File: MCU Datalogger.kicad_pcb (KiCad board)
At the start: 2 copper layers, 50.9 x 30.2 mm, 29 parts, among them J1 Conn_01x04_Pin, J2 Conn_01x09_Pin, J3 Conn_01x04_Pin, J4 Conn_02x03_Odd_Even, U1 24LC1025, U2 24LC1025, U3 DS1337S_, U4 ATMEGA328P-AU, Y1 32.768 KHz, Y2 16 MHz

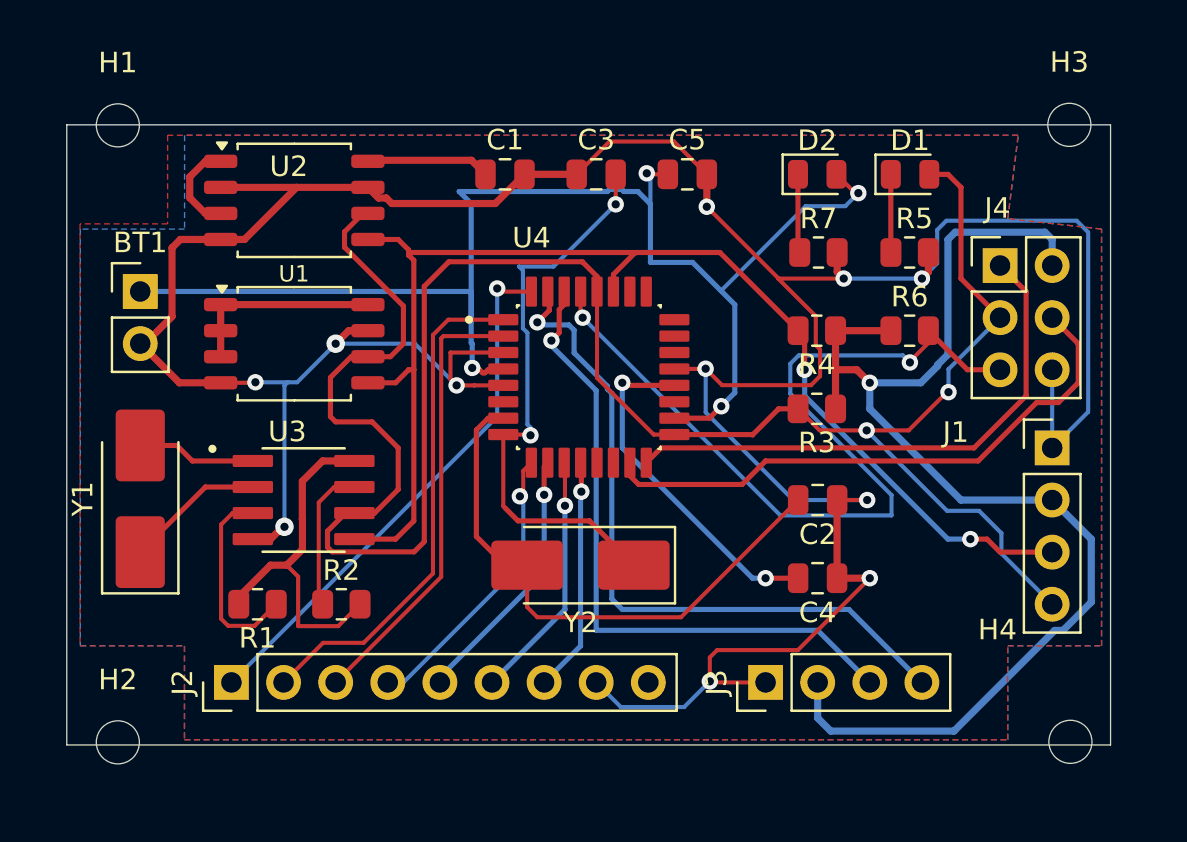
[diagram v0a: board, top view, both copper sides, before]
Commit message: Refined Routing Completed
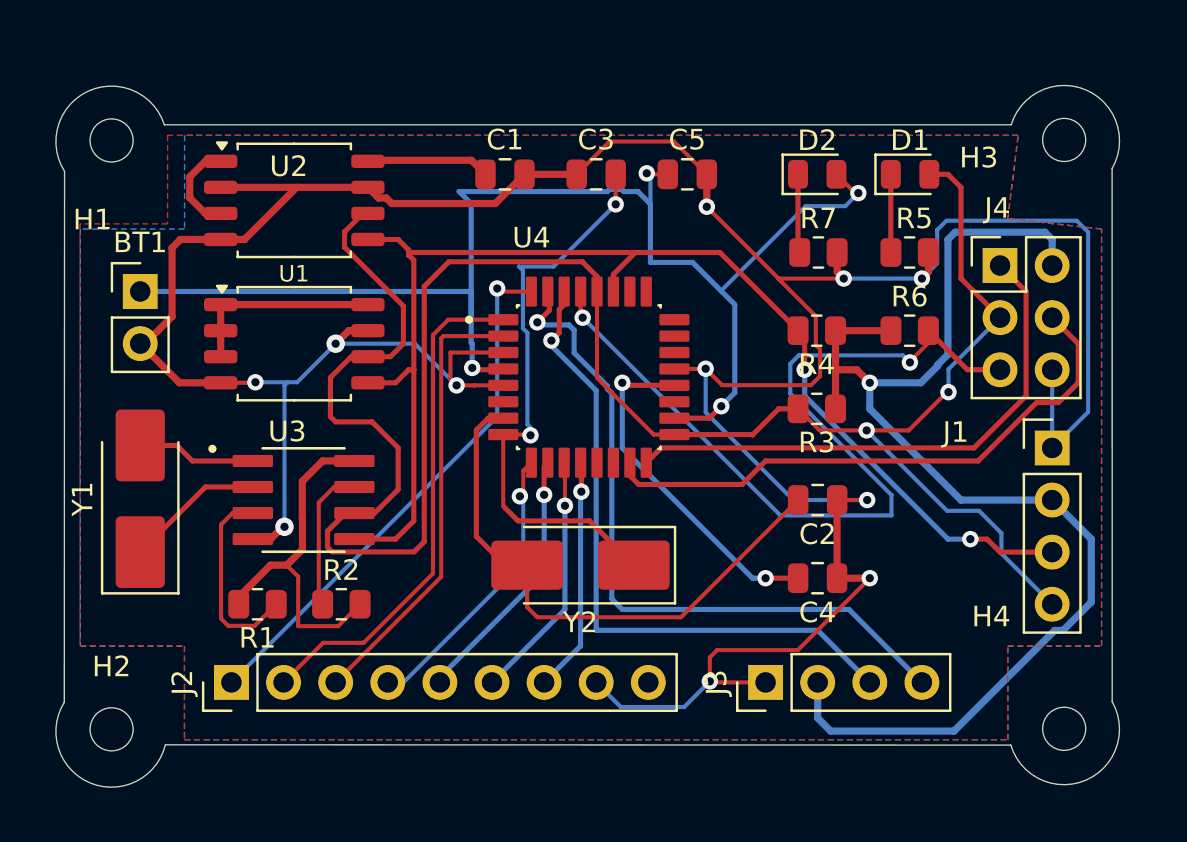
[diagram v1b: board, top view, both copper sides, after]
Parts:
- moved H1 0.80 mm to (66.5, 68.8)
- moved H3 0.78 mm to (113.0, 68.8)
- moved H2 0.70 mm to (66.5, 97.5)
- moved H4 0.70 mm to (113.0, 97.5)
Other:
- board size 50.9 x 30.2 mm -> 51.8 x 34.2 mm
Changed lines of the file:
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@@
 	(footprint "MountingHole:MountingHole_2.1mm"
 		(layer "F.Cu")
-		(at 66.8528 98.171)
+		(at 66.548 97.536)
 		(descr "Mounting Hole 2.1mm, no annular, generated by kicad-footprint-generator mountinghole.py")
 		(tags "mountinghole")
@@
 	(footprint "MountingHole:MountingHole_2.1mm"
 		(layer "F.Cu")
-		(at 113.284 98.1456)
+		(at 112.9792 97.5106)
 		(descr "Mounting Hole 2.1mm, no annular, generated by kicad-footprint-generator mountinghole.py")
 		(tags "mountinghole")
@@
 	(footprint "MountingHole:MountingHole_2.1mm"
 		(layer "F.Cu")
-		(at 66.8528 68.0974)
+		(at 66.548 68.834)
 		(descr "Mounting Hole 2.1mm, no annular, generated by kicad-footprint-generator mountinghole.py")
 		(tags "mountinghole")
 		(property "Reference" "H1"
-			(at 0 -3.05 0)
+			(at -0.928 3.866 0)
 			(layer "F.SilkS")
 			(effects
@@
 	(footprint "MountingHole:MountingHole_2.1mm"
 		(layer "F.Cu")
-		(at 113.2332 68.072)
+		(at 112.9792 68.8086)
 		(descr "Mounting Hole 2.1mm, no annular, generated by kicad-footprint-generator mountinghole.py")
 		(tags "mountinghole")
 		(property "Reference" "H3"
-			(at 0 -3.05 0)
+			(at -4.1592 0.8714 0)
 			(layer "F.SilkS")
 			(effects
@@
 		)
 	)
-	(gr_rect
-		(start 64.3636 68.072)
-		(end 115.240201 98.298)
+	(gr_line
+		(start 64.242154 96.219477)
+		(end 64.254954 70.341677)
+		(stroke
+			(width 0.05)
+			(type default)
+		)
+		(layer "Edge.Cuts")
+	)
+	(gr_arc
+		(start 64.254954 70.341677)
+		(mid 65.394627 66.437058)
+		(end 69.12 68.07)
+		(stroke
+			(width 0.05)
+			(type default)
+		)
+		(layer "Edge.Cuts")
+	)
+	(gr_arc
+		(start 69.17 98.29)
+		(mid 65.491502 100.145426)
+		(end 64.242152 96.219477)
+		(stroke
+			(width 0.05)
+			(type default)
+		)
+		(layer "Edge.Cuts")
+	)
+	(gr_line
+		(start 110.378307 98.305384)
+		(end 69.169999 98.29)
+		(stroke
+			(width 0.05)
+			(type default)
+		)
+		(layer "Edge.Cuts")
+	)
+	(gr_line
+		(start 115.316 70.2)
+		(end 115.32 96.190002)
+		(stroke
+			(width 0.05)
+			(type default)
+		)
+		(layer "Edge.Cuts")
+	)
+	(gr_line
+		(start 69.12 68.070003)
+		(end 110.396855 68.071052)
+		(stroke
+			(width 0.05)
+			(type default)
+		)
+		(layer "Edge.Cuts")
+	)
+	(gr_arc
+		(start 110.396855 68.071052)
+		(mid 114.051623 66.37391)
+		(end 115.316 70.2)
+		(stroke
+			(width 0.05)
+			(type default)
+		)
+		(layer "Edge.Cuts")
+	)
+	(gr_arc
+		(start 115.32 96.19)
+		(mid 114.034573 100.016923)
+		(end 110.378305 98.305384)
 		(stroke
 			(width 0.05)
 			(type default)
 		)
-		(fill no)
 		(layer "Edge.Cuts")
 	)
@@
 	)
 	(segment
-		(start 84.629801 80.159401)
-		(end 84.747221 80.159401)
+		(start 84.2148 80.01)
+		(end 85.6 80.01)
 		(width 0.25)
 		(layer "F.Cu")
@@
 	)
 	(segment
-		(start 84.4804 80.01)
-		(end 84.629801 80.159401)
-		(width 0.25)
-		(layer "F.Cu")
-		(net 1)
-	)
-	(segment
-		(start 84.2148 80.01)
-		(end 84.4804 80.01)
-		(width 0.25)
-		(layer "F.Cu")
-		(net 1)
-	)
-	(segment
-		(start 84.747221 80.159401)
-		(end 84.896622 80.01)
-		(width 0.25)
-		(layer "F.Cu")
-		(net 1)
-	)
-	(segment
 		(start 85.6 80.01)
 		(end 85.64 79.97)
@@
 	)
 	(segment
-		(start 84.896622 80.01)
-		(end 85.6 80.01)
-		(width 0.25)
-		(layer "F.Cu")
-		(net 1)
-	)
-	(segment
 		(start 92.6846 70.485)
 		(end 92.6338 70.4342)
@@
 	)
 	(segment
-		(start 90.932 91.186)
-		(end 91.44 91.694)
+		(start 87.4268 77.8256)
+		(end 88.83848 77.8256)
 		(width 0.25)
 		(layer "B.Cu")
@@
 	)
 	(segment
-		(start 87.2998 77.6986)
-		(end 87.4268 77.8256)
-		(width 0.25)
-		(layer "B.Cu")
-		(net 19)
-	)
-	(segment
-		(start 87.4268 77.8256)
-		(end 88.83848 77.8256)
+		(start 90.932 91.186)
+		(end 91.44 91.694)
 		(width 0.25)
 		(layer "B.Cu")
@@
 	)
 	(segment
-		(start 91.44 91.694)
-		(end 102.489 91.694)
+		(start 87.2998 77.6986)
+		(end 87.4268 77.8256)
 		(width 0.25)
 		(layer "B.Cu")
@@
 	)
 	(segment
-		(start 89.0926 79.18497)
-		(end 90.714 80.80637)
+		(start 102.489 91.694)
+		(end 106.045 95.25)
 		(width 0.25)
 		(layer "B.Cu")
@@
 	)
 	(segment
-		(start 102.489 91.694)
-		(end 106.045 95.25)
+		(start 90.932 81.16372)
+		(end 90.932 91.186)
 		(width 0.25)
 		(layer "B.Cu")
@@
 	)
 	(segment
-		(start 90.932 81.16372)
-		(end 90.932 91.186)
+		(start 91.44 91.694)
+		(end 102.489 91.694)
+		(width 0.25)
+		(layer "B.Cu")
+		(net 19)
+	)
+	(segment
+		(start 89.0926 79.18497)
+		(end 90.714 80.80637)
 		(width 0.25)
 		(layer "B.Cu")

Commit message: Version for manufacturing
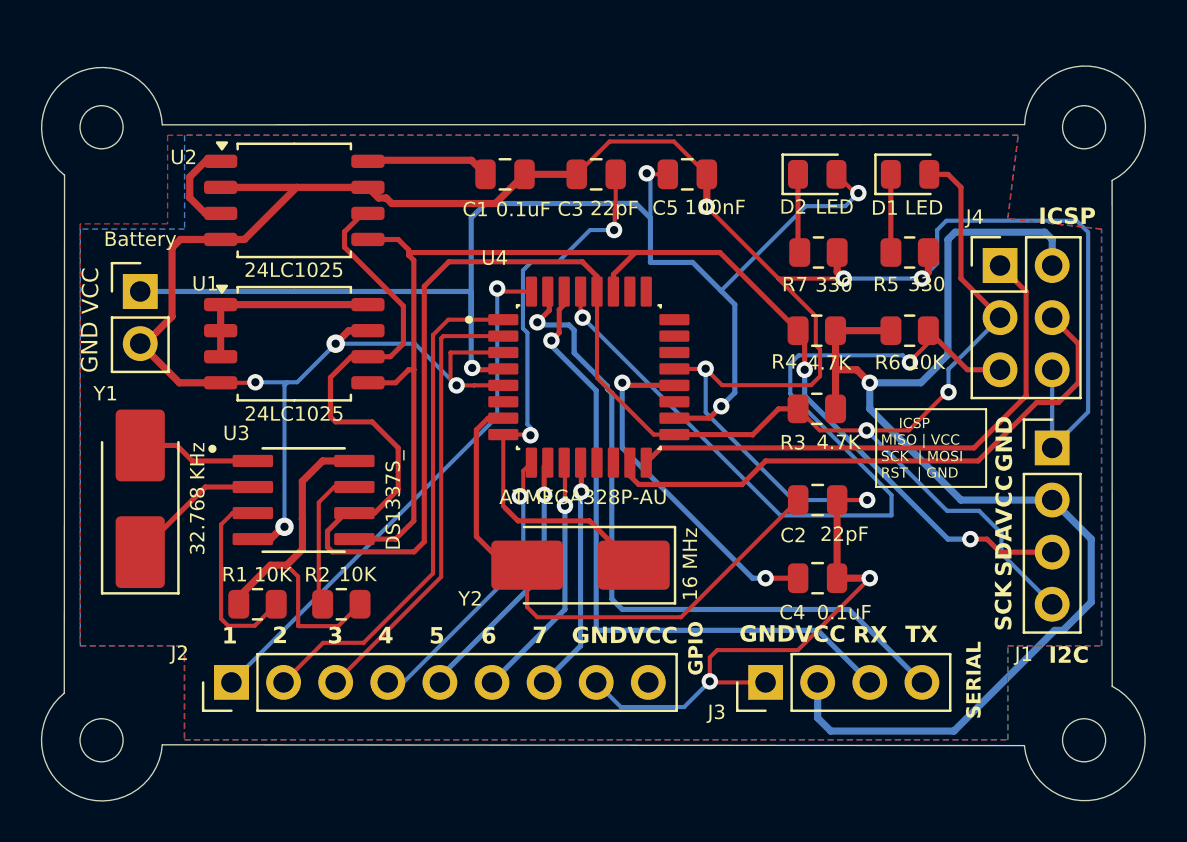
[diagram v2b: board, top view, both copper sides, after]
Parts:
- added REF**: KiCad-Logo2_5mm_SilkScreen, Symbol:KiCad-Logo2_5mm_SilkScreen, B.Cu at (75.9, 72.2)
- moved H3 1.15 mm to (114.0, 68.2)
- moved H4 1.12 mm to (114.0, 98.1)
- moved H1 0.81 mm to (66.1, 68.2)
- moved H2 0.72 mm to (66.1, 98.1)
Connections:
- BT1 pad 1: Net-(BT1-+) -> /Vcc
- C5 pad 1: Net-(BT1-+) -> /Vcc
- D2 pad 2: Net-(BT1-+) -> /Vcc
- U4 pad 18: Net-(BT1-+) -> /Vcc
- U4 pad 4: Net-(BT1-+) -> /Vcc
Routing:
- net Net-(BT1-+): track 68.8 -> 0.00 mm, vias 4 -> 0
- net /Vcc: track 98.6 -> 164.9 mm, vias 1 -> 5
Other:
- board size 51.8 x 34.2 mm -> 53.8 x 35.8 mm
- board text added: "- 2Mbit EEPROM - RTC - I2C, SPI, GPIOs"
- board text added: "1"
- board text added: "2"
- board text added: "3"
- board text added: "4"
- board text added: "5"
- board text added: "6"
- board text added: "7"
- board text added: "Data Logger with ATMega328P"
- board text added: "GND"
- board text added: "GPIO"
- board text added: "I2C"
- board text added: "ICSP"
- board text added: "ICSP MISO | VCC SCK | MOSI RST | GND"
- board text added: "JP Electronics Oct-2025"
- board text added: "RX"
- board text added: "SCK"
- board text added: "SDA"
- board text added: "SERIAL"
- board text added: "TX"
- board text added: "VCC"

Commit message: Completed 2-layer PCB project
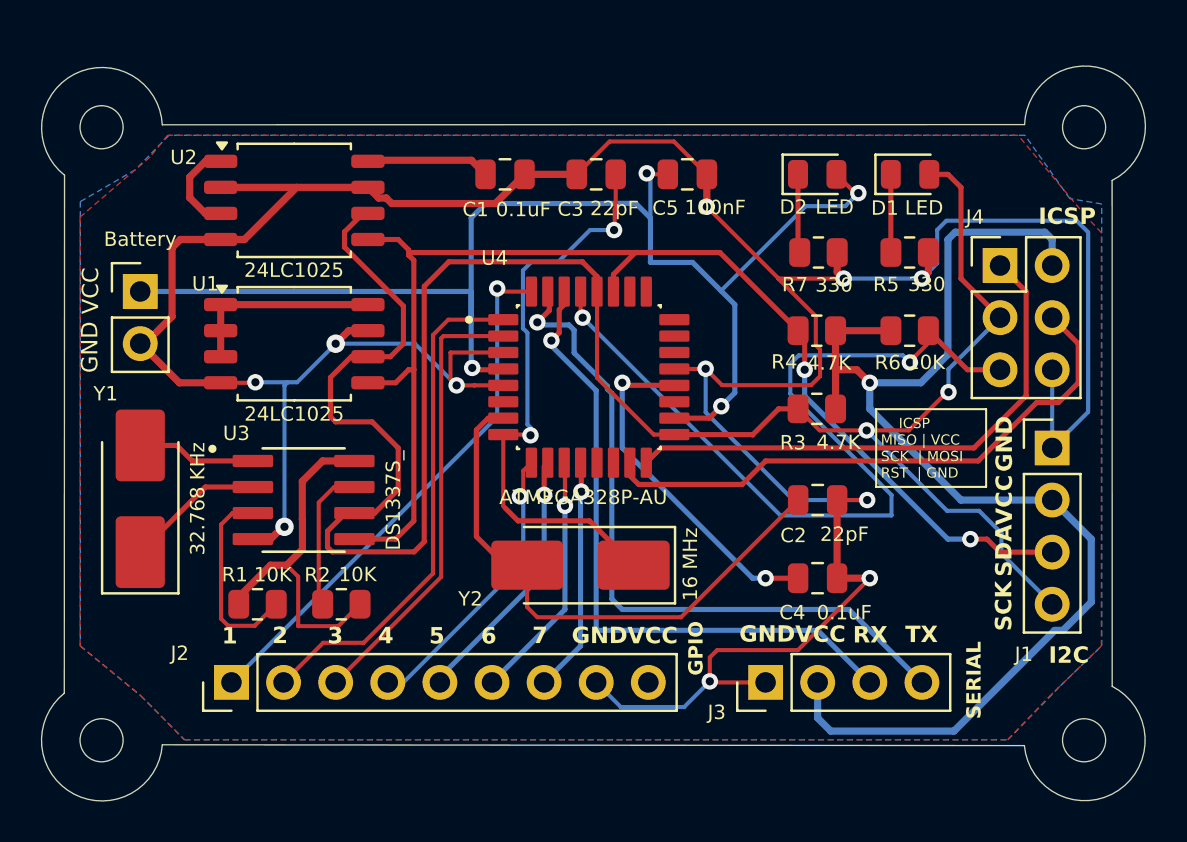
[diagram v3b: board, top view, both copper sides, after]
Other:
- board text added: "0.2000 mm / 0.0000 mm"
- board text added: "0.3000 mm"
- board text added: "1.6000 mm"
- board text added: "53.8097 mm x 35.8235 mm"
- board text added: "BOARD CHARACTERISTICS"
- board text added: "Board Thickness:"
- board text added: "Board overall dimensions:"
- board text added: "Castellated pads:"
- board text added: "Copper Finish:"
- board text added: "Copper Layer Count:"
- board text added: "Edge card connectors:"
- board text added: "Impedance Control:"
- board text added: "Min hole diameter:"
- board text added: "Min track/spacing:"
- board text added: "No"
- board text added: "None"
- board text added: "Plated Board Edge:"
